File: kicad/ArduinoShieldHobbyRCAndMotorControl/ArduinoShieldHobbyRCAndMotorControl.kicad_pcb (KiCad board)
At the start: 2 copper layers, 68.6 x 53.3 mm, 15 parts, among them J1 Power, J10 Conn_01x03_Socket, J11 Conn_01x03_Socket, J2 Digital/PWM, J3 Analog, J4 Digital/PWM, J5 Conn_01x03_Socket, J6 Conn_01x07_Pin, J7 Conn_01x03_Socket, J8 Conn_01x03_Socket, J9 Conn_01x03_Socket

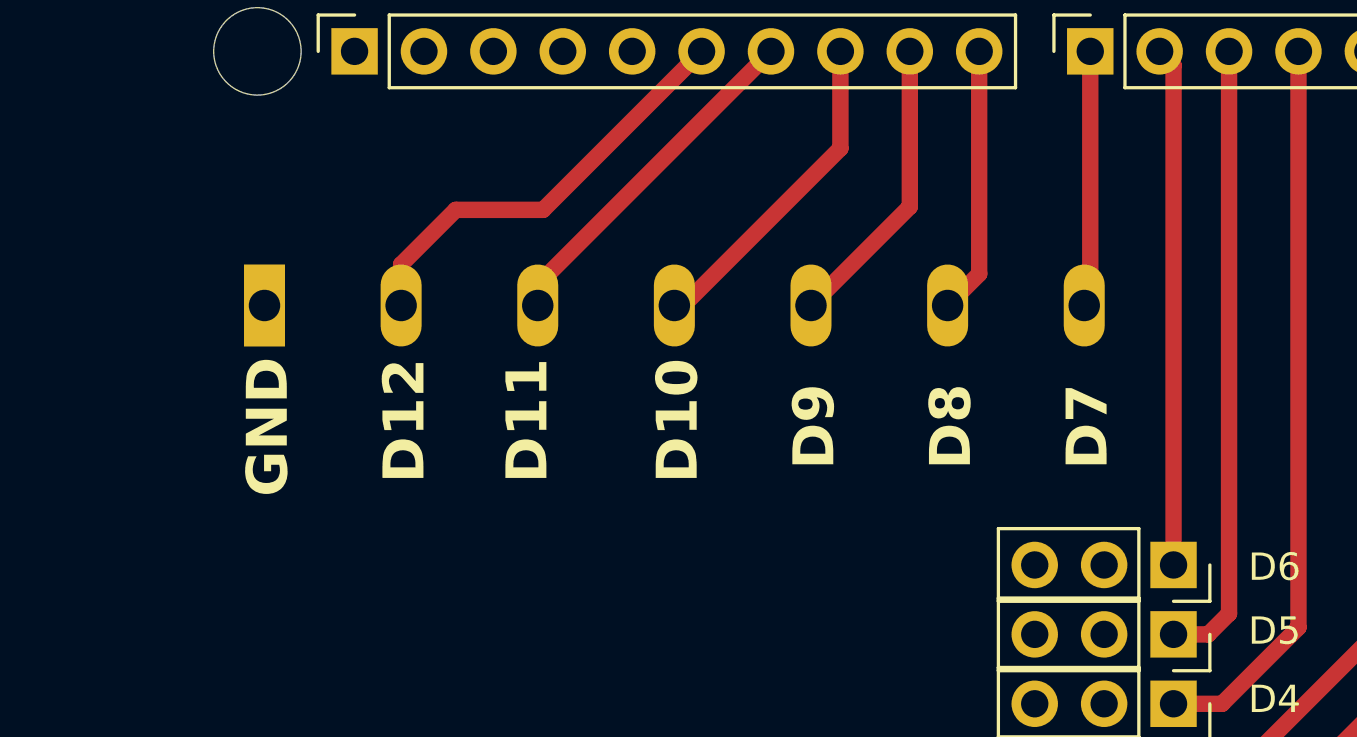
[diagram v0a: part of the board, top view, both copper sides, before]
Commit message: minor changes for Machine Lab 2026
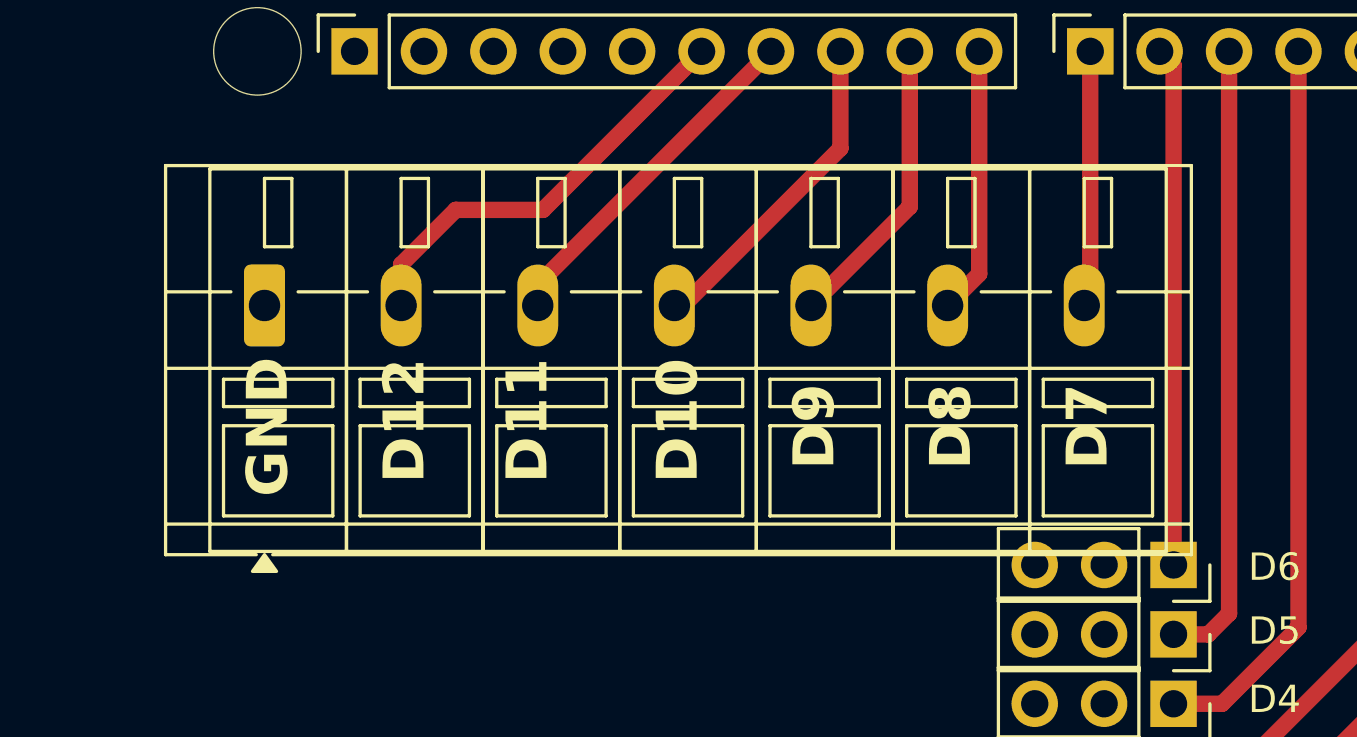
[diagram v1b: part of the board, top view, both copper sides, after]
